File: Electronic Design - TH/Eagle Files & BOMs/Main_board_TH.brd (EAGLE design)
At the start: 90 x 137.2 mm, 41 parts, among them M1 ARDUINO-NANO-3.0, Q1 IRF9520, Q2 IRF9520

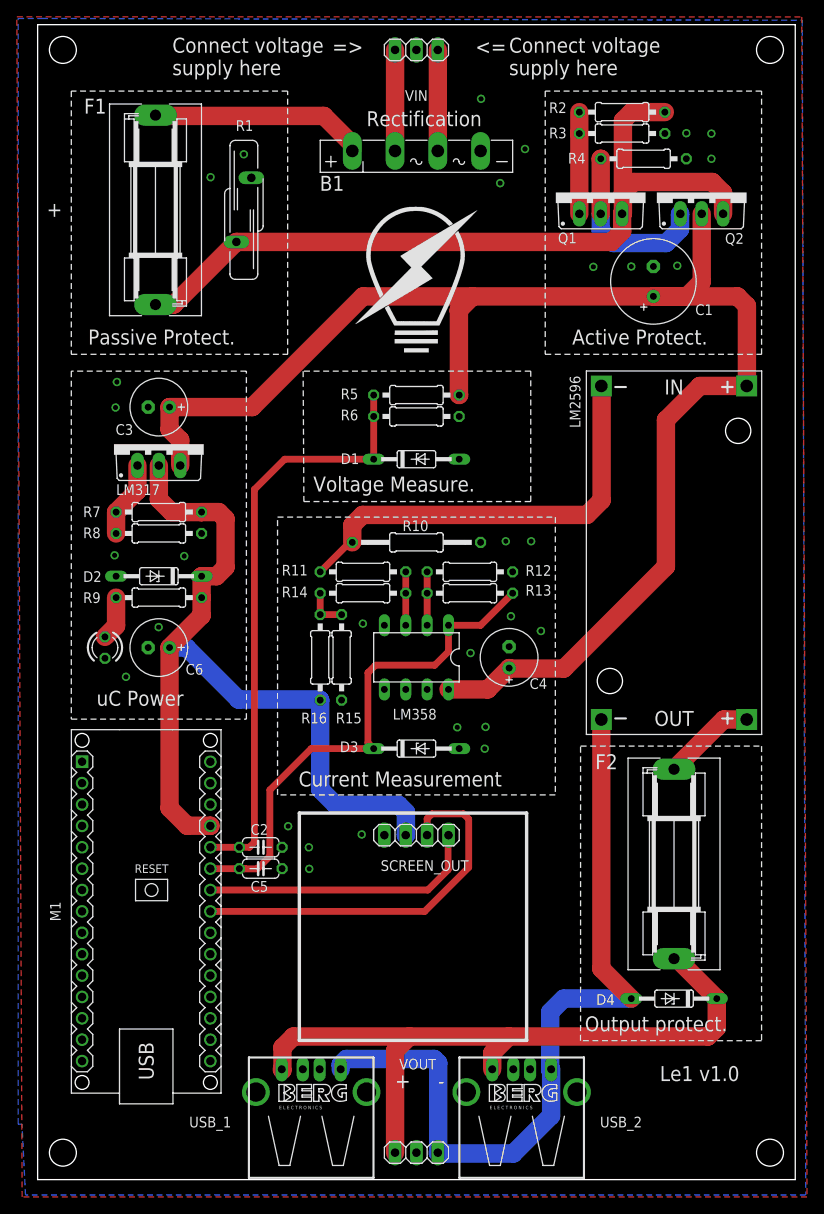
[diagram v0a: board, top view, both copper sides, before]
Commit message: minor cosmetic changes in the silkscreen layer
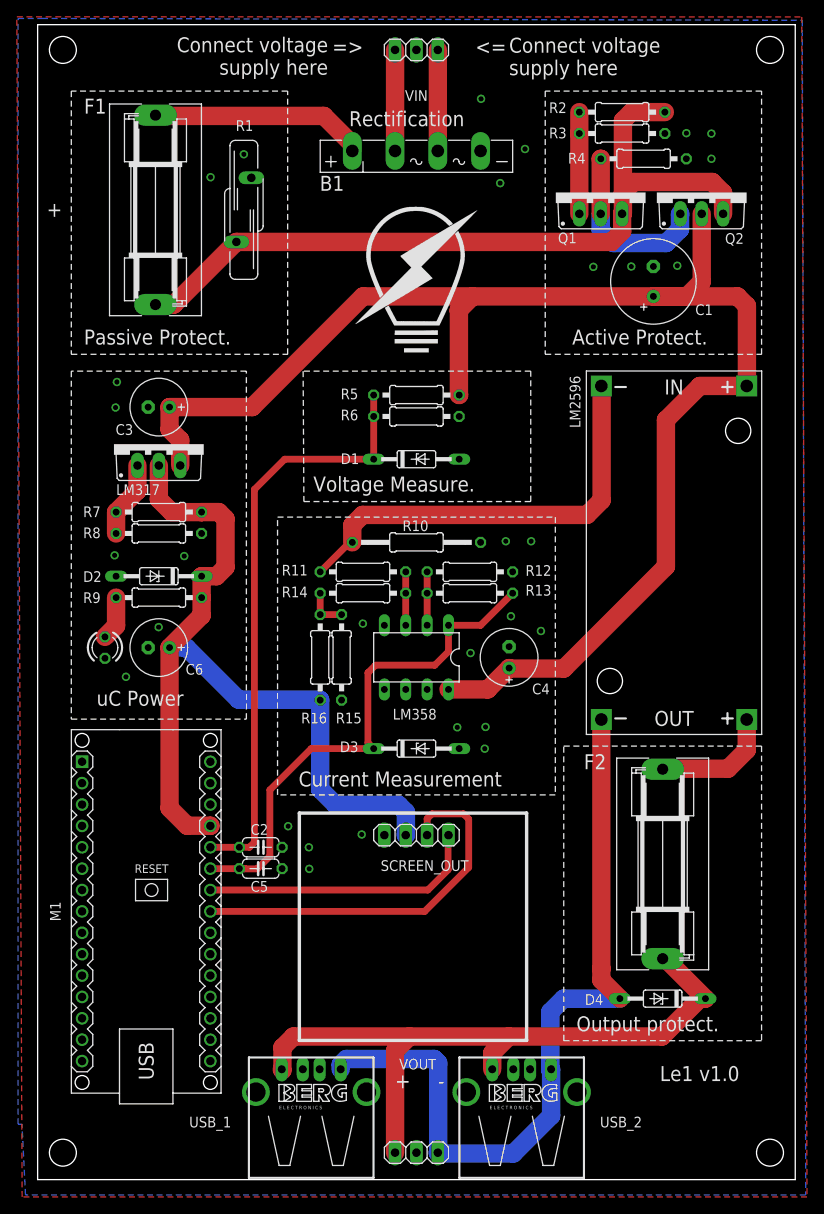
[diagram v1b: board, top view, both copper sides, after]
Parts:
- moved D4 1.35 mm to (74.2, 21.3)
- moved F2 1.35 mm to (74.2, 37.3)
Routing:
- net VOUT_PREFUSE: track 11.1 -> 16.9 mm
- net VOUT_FINAL: track 85.1 -> 81.8 mm
- net N$10: track 96.1 -> 94.2 mm
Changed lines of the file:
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@@
 <wire x1="31.09" y1="16.34" x2="58.09" y2="16.34" width="0.4064" layer="21"/>
 <wire x1="58.09" y1="16.34" x2="58.09" y2="43.34" width="0.4064" layer="21"/>
-<text x="16" y="131" size="1.778" layer="25">Connect voltage
+<text x="34.5" y="135.5" size="1.778" layer="25" rot="R180">Connect voltage
 supply here </text>
 <wire x1="29.7" y1="129.11" x2="4" y2="129.11" width="0.15" layer="21" style="shortdash"/>
@@
 <wire x1="29.7" y1="97.84" x2="29.7" y2="129.11" width="0.15" layer="21" style="shortdash"/>
 <text x="52" y="133.5" size="1.778" layer="25">&lt;=</text>
-<text x="39.0672" y="124.9396" size="1.778" layer="25">Rectification</text>
-<text x="6" y="99" size="1.778" layer="25">Passive Protect.</text>
+<text x="37" y="124.9396" size="1.778" layer="25">Rectification</text>
+<text x="5.5" y="99" size="1.778" layer="25">Passive Protect.</text>
 <text x="63.5" y="99" size="1.778" layer="25">Active Protect.</text>
 <wire x1="61.5" y1="45.5" x2="28.5" y2="45.5" width="0.15" layer="21" style="shortdash"/>
@@
 <text x="32.75" y="81.54" size="1.778" layer="25">Voltage Measure.</text>
 <text x="31" y="46.5" size="1.778" layer="25">Current Measurement</text>
-<wire x1="86" y1="16.3" x2="64.5" y2="16.3" width="0.15" layer="21" style="shortdash"/>
-<wire x1="64.5" y1="16.3" x2="64.5" y2="51.3" width="0.15" layer="21" style="shortdash"/>
-<wire x1="64.5" y1="51.3" x2="86" y2="51.3" width="0.15" layer="21" style="shortdash"/>
+<wire x1="86" y1="16.3" x2="62.5" y2="16.3" width="0.15" layer="21" style="shortdash"/>
+<wire x1="62.5" y1="16.3" x2="62.5" y2="51.3" width="0.15" layer="21" style="shortdash"/>
+<wire x1="62.5" y1="51.3" x2="86" y2="51.3" width="0.15" layer="21" style="shortdash"/>
 <wire x1="86" y1="51.3" x2="86" y2="16.3" width="0.15" layer="21" style="shortdash"/>
-<text x="65" y="17.42" size="1.778" layer="25">Output protect.</text>
+<text x="64" y="17.42" size="1.778" layer="25">Output protect.</text>
 <text x="42.46" y="10.65" size="1.778" layer="25">+</text>
 <text x="47.54" y="10.65" size="1.778" layer="25">-</text>
@@
 <attribute name="VALUE" x="42.46" y="130.825" size="1.27" layer="27"/>
 </element>
-<element name="F2" library="fuse" package="SH22,5A" value="FUSESH22,5A" x="75.6" y="37.3" smashed="yes" rot="R270">
-<attribute name="MF" value="" x="75.6" y="37.3" size="1.778" layer="27" rot="R270" display="off"/>
-<attribute name="MPN" value="" x="75.6" y="37.3" size="1.778" layer="27" rot="R270" display="off"/>
-<attribute name="OC_NEWARK" value="unknown" x="75.6" y="37.3" size="1.778" layer="27" rot="R270" display="off"/>
-<attribute name="OC_FARNELL" value="unknown" x="75.6" y="37.3" size="1.778" layer="27" rot="R270" display="off"/>
-<attribute name="NAME" x="66.24" y="48.55" size="1.778" layer="25" ratio="10"/>
-<attribute name="VALUE" x="67.98" y="37.2746" size="1.778" layer="27" ratio="10" rot="R270"/>
+<element name="F2" library="fuse" package="SH22,5A" value="FUSESH22,5A" x="74.25" y="37.3" smashed="yes" rot="R270">
+<attribute name="MF" value="" x="74.25" y="37.3" size="1.778" layer="27" rot="R270" display="off"/>
+<attribute name="MPN" value="" x="74.25" y="37.3" size="1.778" layer="27" rot="R270" display="off"/>
+<attribute name="OC_NEWARK" value="unknown" x="74.25" y="37.3" size="1.778" layer="27" rot="R270" display="off"/>
+<attribute name="OC_FARNELL" value="unknown" x="74.25" y="37.3" size="1.778" layer="27" rot="R270" display="off"/>
+<attribute name="NAME" x="64.89" y="48.55" size="1.778" layer="25" ratio="10"/>
+<attribute name="VALUE" x="66.63" y="37.2746" size="1.778" layer="27" ratio="10" rot="R270"/>
 </element>
 <element name="D1" library="diode" package="DO35Z10" value="5.1V" x="45" y="85.38" smashed="yes">
@@
 <attribute name="VALUE" x="16.686" y="74.02" size="1.27" layer="27" ratio="10" rot="R180"/>
 </element>
-<element name="D4" library="diode" package="DO35Z10" value="5.1V" x="75.6" y="21.3" smashed="yes" rot="R180">
-<attribute name="NAME" x="68.556" y="21.83" size="1.27" layer="25" ratio="10" rot="R180"/>
-<attribute name="VALUE" x="77.886" y="23.84" size="1.27" layer="27" ratio="10" rot="R180"/>
+<element name="D4" library="diode" package="DO35Z10" value="5.1V" x="74.25" y="21.3" smashed="yes" rot="R180">
+<attribute name="NAME" x="67.206" y="21.83" size="1.27" layer="25" ratio="10" rot="R180"/>
+<attribute name="VALUE" x="76.536" y="23.84" size="1.27" layer="27" ratio="10" rot="R180"/>
 </element>
 <element name="UC_PWR" library="led" package="LED3MM" value="" x="8" y="63" smashed="yes" rot="R270">
@@
 </element>
 <element name="C4" library="resistor" package="E2,5-7" value="10u" x="56.01" y="61.84" smashed="yes" rot="R90">
-<attribute name="NAME" x="58.438" y="58.092" size="1.27" layer="25" ratio="10"/>
+<attribute name="NAME" x="58.7428" y="57.457" size="1.27" layer="25" ratio="10"/>
 <attribute name="VALUE" x="59.185" y="64.888" size="1.27" layer="27" ratio="10" rot="R90"/>
 </element>
@@
 <contactref element="F2" pad="2"/>
 <contactref element="VOUT" pad="1"/>
-<wire x1="75.6" y1="26.0478" x2="75.9322" y2="26.0478" width="2.1844" layer="1"/>
-<wire x1="75.9322" y1="26.0478" x2="80.68" y2="21.3" width="2.1844" layer="1"/>
 <contactref element="USB_1" pad="1"/>
 <contactref element="USB_2" pad="1"/>
-<wire x1="80.68" y1="21.3" x2="80.68" y2="17.84" width="2.1844" layer="1"/>
-<wire x1="80.68" y1="17.84" x2="79.64" y2="16.8" width="2.1844" layer="1"/>
-<wire x1="55.97" y1="16.8" x2="79.64" y2="16.8" width="2.1844" layer="1"/>
 <wire x1="44.17" y1="16.8" x2="55.97" y2="16.8" width="2.1844" layer="1"/>
 <wire x1="44.17" y1="16.8" x2="30.38" y2="16.8" width="2.1844" layer="1"/>
@@
 <wire x1="42.46" y1="3" x2="42.46" y2="15.09" width="2.1844" layer="1"/>
 <wire x1="42.46" y1="15.09" x2="44.17" y2="16.8" width="2.1844" layer="1"/>
+<wire x1="74.18" y1="16.8" x2="55.97" y2="16.8" width="2.1844" layer="1"/>
+<wire x1="74.25" y1="26.0478" x2="74.5822" y2="26.0478" width="2.1844" layer="1"/>
+<wire x1="74.5822" y1="26.0478" x2="79.33" y2="21.3" width="2.1844" layer="1"/>
+<wire x1="79.33" y1="21.3" x2="78.68" y2="21.3" width="2.1844" layer="1"/>
+<wire x1="78.68" y1="21.3" x2="74.18" y2="16.8" width="2.1844" layer="1"/>
 </signal>
 <signal name="VOUT_PREFUSE">
 <contactref element="F2" pad="1"/>
 <contactref element="LM2596" pad="OUT+"/>
-<wire x1="84.236" y1="54.458" x2="81.5058" y2="54.458" width="2.1844" layer="1"/>
-<wire x1="81.5058" y1="54.458" x2="75.6" y2="48.5522" width="2.1844" layer="1"/>
+<wire x1="84.236" y1="54.458" x2="84.236" y2="50.835" width="2.1844" layer="1"/>
+<wire x1="84.236" y1="50.835" x2="82.0166" y2="48.6156" width="2.1844" layer="1"/>
+<wire x1="82.0166" y1="48.6156" x2="73.0634" y2="48.6156" width="2.1844" layer="1"/>
+<wire x1="73.0634" y1="48.6156" x2="74.25" y2="48.5522" width="2.1844" layer="1"/>
 </signal>
 <signal name="GND1">
@@
 <contactref element="LM2596" pad="OUT-"/>
 <wire x1="66.964" y1="54.458" x2="66.964" y2="24.856" width="2.1844" layer="1"/>
-<wire x1="66.964" y1="24.856" x2="70.52" y2="21.3" width="2.1844" layer="1"/>
 <contactref element="USB_1" pad="4"/>
 <contactref element="USB_2" pad="4"/>
@@
 <wire x1="47.59" y1="13.65" x2="47.59" y2="3.05" width="2.1844" layer="16"/>
 <wire x1="47.54" y1="3" x2="47.59" y2="3.05" width="2.1844" layer="16"/>
-<wire x1="70.52" y1="21.3" x2="62.48" y2="21.3" width="2.1844" layer="16"/>
+<wire x1="69.17" y1="21.3" x2="62.48" y2="21.3" width="2.1844" layer="16"/>
 <wire x1="62.48" y1="21.3" x2="60.9" y2="19.72" width="2.1844" layer="16"/>
 <wire x1="60.9" y1="19.72" x2="60.9" y2="12.81" width="2.1844" layer="16"/>
@@
 <wire x1="56.52" y1="2.9" x2="47.64" y2="2.9" width="2.1844" layer="16"/>
 <wire x1="47.64" y1="2.9" x2="47.54" y2="3" width="2.1844" layer="16"/>
+<wire x1="66.9798" y1="24.8402" x2="66.964" y2="24.856" width="2.1844" layer="1"/>
+<wire x1="66.964" y1="24.856" x2="66.964" y2="23.506" width="2.1844" layer="1"/>
+<wire x1="66.964" y1="23.506" x2="69.17" y2="21.3" width="2.1844" layer="1"/>
 </signal>
 <signal name="A5">
